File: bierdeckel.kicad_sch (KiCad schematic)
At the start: 27 parts, among them J1 Pogo, J2 Pogo, J3 Pogo, J4 Pogo, Q1 BSS138P,215, SW1 PTS526 SK15 SMTR2 LFS, SW2 PTS526 SK15 SMTR2 LFS, SW3 PTS526 SK15 SMTR2 LFS, U1 ESP32-C3-WROOM-02, U5 ESP32-C3-MINI-1

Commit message: further work
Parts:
- C3: footprint Capacitor_SMD:C_0805_2012Metric -> Capacitor_SMD:C_0603_1608Metric
- R1, R2, R3, R4, R5, R6, R7: footprint Resistor_SMD:R_0805_2012Metric -> Resistor_SMD:R_0603_1608Metric
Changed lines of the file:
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@@
 			)
 		)
-		(property "Footprint" "Resistor_SMD:R_0805_2012Metric"
+		(property "Footprint" "Resistor_SMD:R_0603_1608Metric"
 			(at 129.54 73.152 90)
 			(effects
@@
 			)
 		)
-		(property "Footprint" "Capacitor_SMD:C_0805_2012Metric"
+		(property "Footprint" "Capacitor_SMD:C_0603_1608Metric"
 			(at 225.7552 53.34 0)
 			(effects
@@
 			)
 		)
-		(property "Footprint" "Resistor_SMD:R_0805_2012Metric"
+		(property "Footprint" "Resistor_SMD:R_0603_1608Metric"
 			(at 121.92 52.832 90)
 			(effects
@@
 			)
 		)
-		(property "Footprint" "Resistor_SMD:R_0805_2012Metric"
+		(property "Footprint" "Resistor_SMD:R_0603_1608Metric"
 			(at 109.728 76.2 90)
 			(effects
@@
 			)
 		)
-		(property "Footprint" "Resistor_SMD:R_0805_2012Metric"
+		(property "Footprint" "Resistor_SMD:R_0603_1608Metric"
 			(at 109.728 60.96 90)
 			(effects
@@
 			)
 		)
-		(property "Footprint" "Resistor_SMD:R_0805_2012Metric"
+		(property "Footprint" "Resistor_SMD:R_0603_1608Metric"
 			(at 146.812 60.96 90)
 			(effects
@@
 			)
 		)
-		(property "Footprint" "Resistor_SMD:R_0805_2012Metric"
+		(property "Footprint" "Resistor_SMD:R_0603_1608Metric"
 			(at 150.368 49.53 90)
 			(effects
@@
 			)
 		)
-		(property "Footprint" "Resistor_SMD:R_0805_2012Metric"
+		(property "Footprint" "Resistor_SMD:R_0603_1608Metric"
 			(at 174.752 52.07 90)
 			(effects

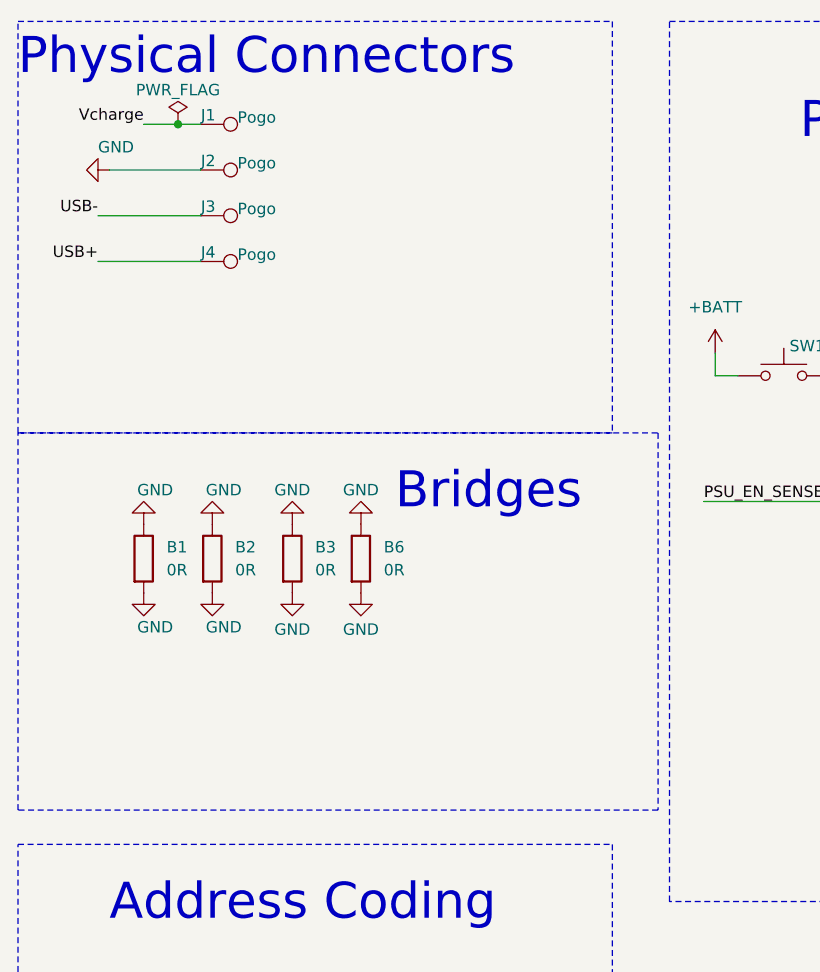
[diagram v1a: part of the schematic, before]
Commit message: before USB connector
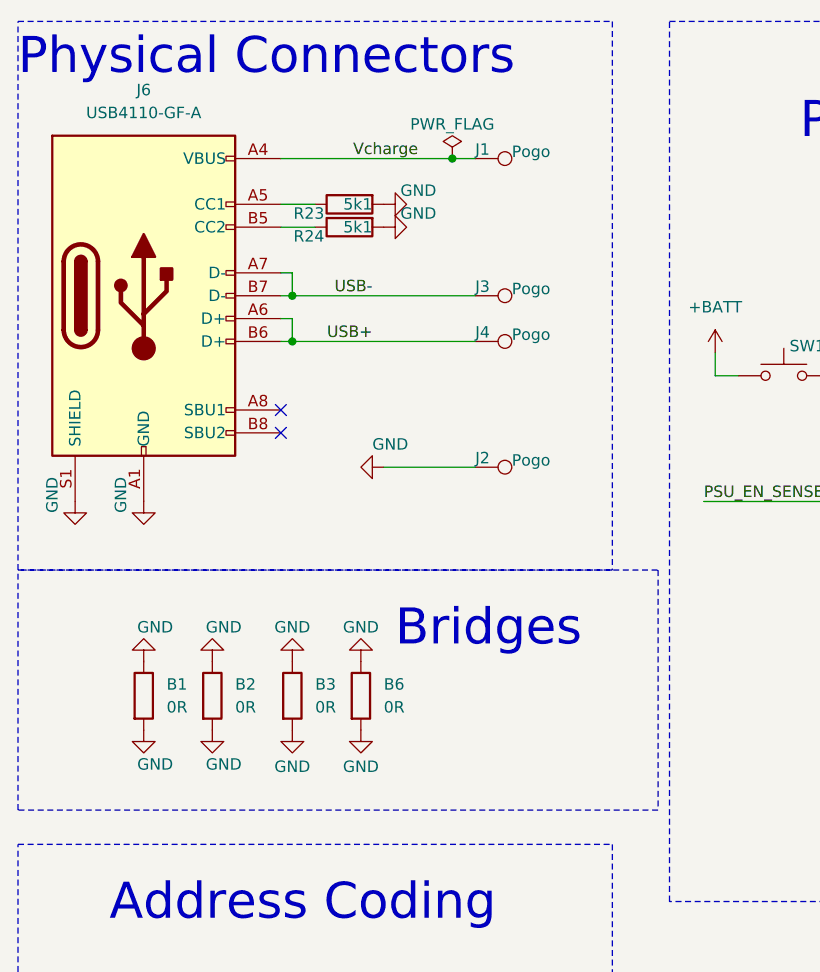
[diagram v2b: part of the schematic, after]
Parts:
- added J6: USB4110-GF-A, Connector_USB:USB_C_Receptacle_GCT_USB4110, symbol Connector:USB_C_Receptacle_USB2.0_16P
- added R23, R24: 5k1, Resistor_SMD:R_0603_1608Metric, symbol Device:R
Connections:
- net GND: now also J6.A1 (GND), J6.A12 (GND), J6.B1 (GND), J6.B12 (GND), J6.S1 (SHIELD), R23.2, R24.2
- net USB+: now also J6.A6 (D+), J6.B6 (D+)
- net USB-: now also J6.A7 (D-), J6.B7 (D-)
- net Vcharge: now also J6.A4 (VBUS), J6.A9 (VBUS), J6.B4 (VBUS), J6.B9 (VBUS)
- new net: J6.A5 (CC1), R23.1
- new net: J6.B5 (CC2), R24.1
- no-connect marks 10 -> 12
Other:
- moved on the sheet: B1, B2, B3, B6, J1, J2, J3, J4
